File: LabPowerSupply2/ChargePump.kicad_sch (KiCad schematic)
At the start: 9 parts, among them Q1_CP1 FMMT495TA

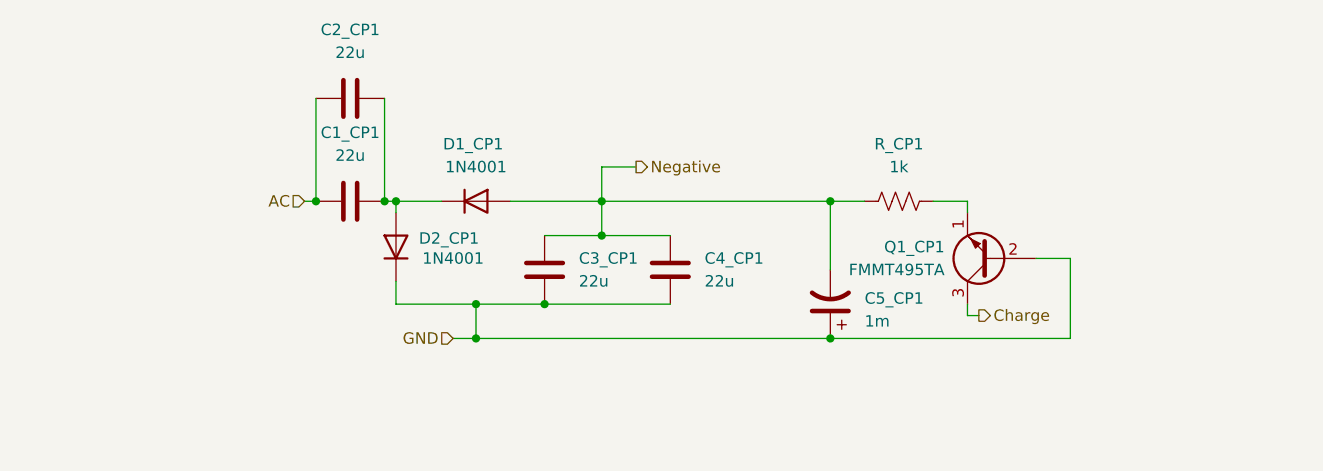
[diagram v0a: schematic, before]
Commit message: Beautifing the Schematic
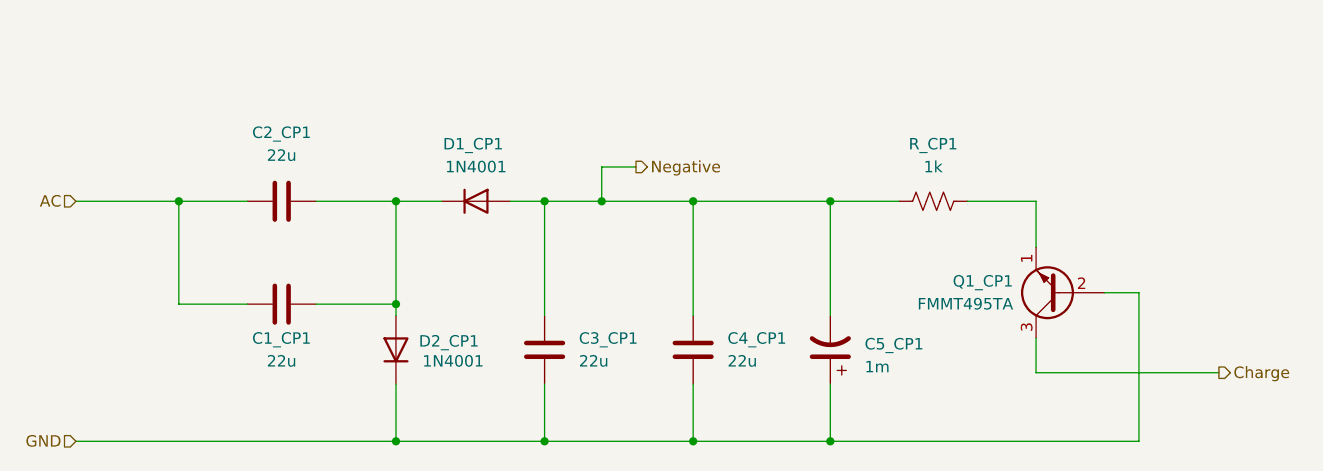
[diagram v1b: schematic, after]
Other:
- moved on the sheet: C1_CP1, C2_CP1, C3_CP1, C4_CP1, C5_CP1, D2_CP1, Q1_CP1, R_CP1
